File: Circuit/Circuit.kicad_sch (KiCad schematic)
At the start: 26 parts, among them J1 Conn_01x08_Socket, J2 Conn_01x08_Socket, Q2 S8050, Q3 S8050, Q4 S8550, Q5 IRFZ44n, SW1 SW_DPDT_x2, SW2 SW_DPDT_x2, U1 L7805

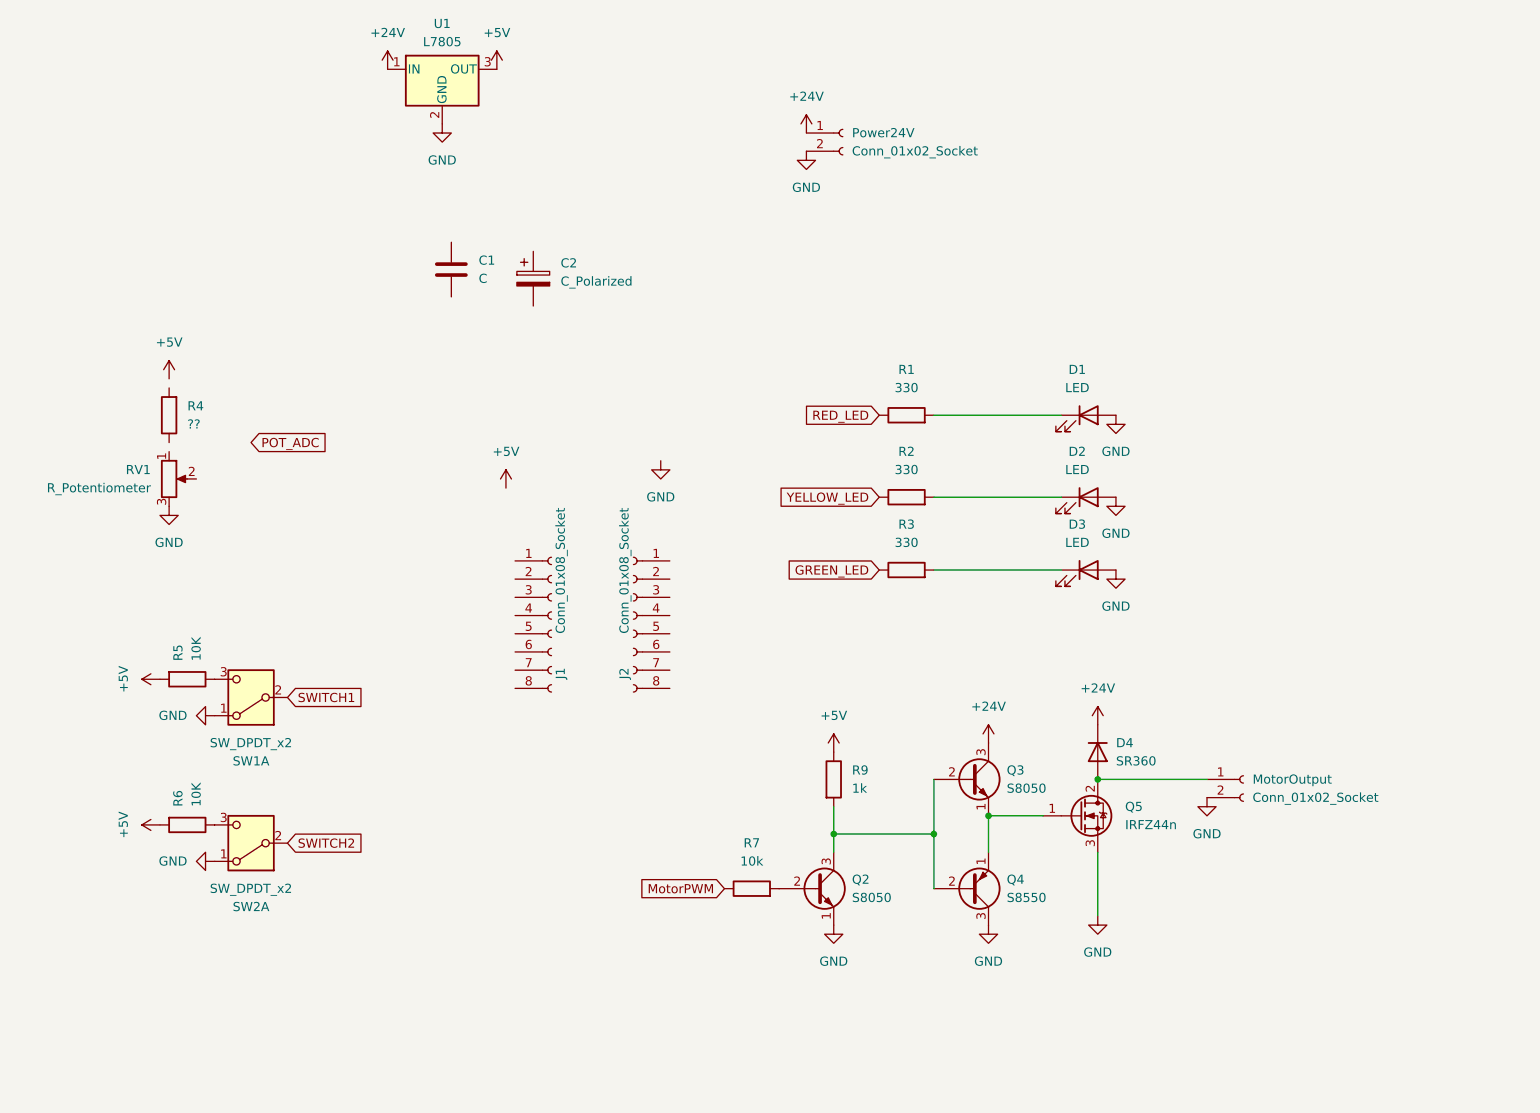
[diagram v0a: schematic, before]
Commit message: finished circuit and started PCB
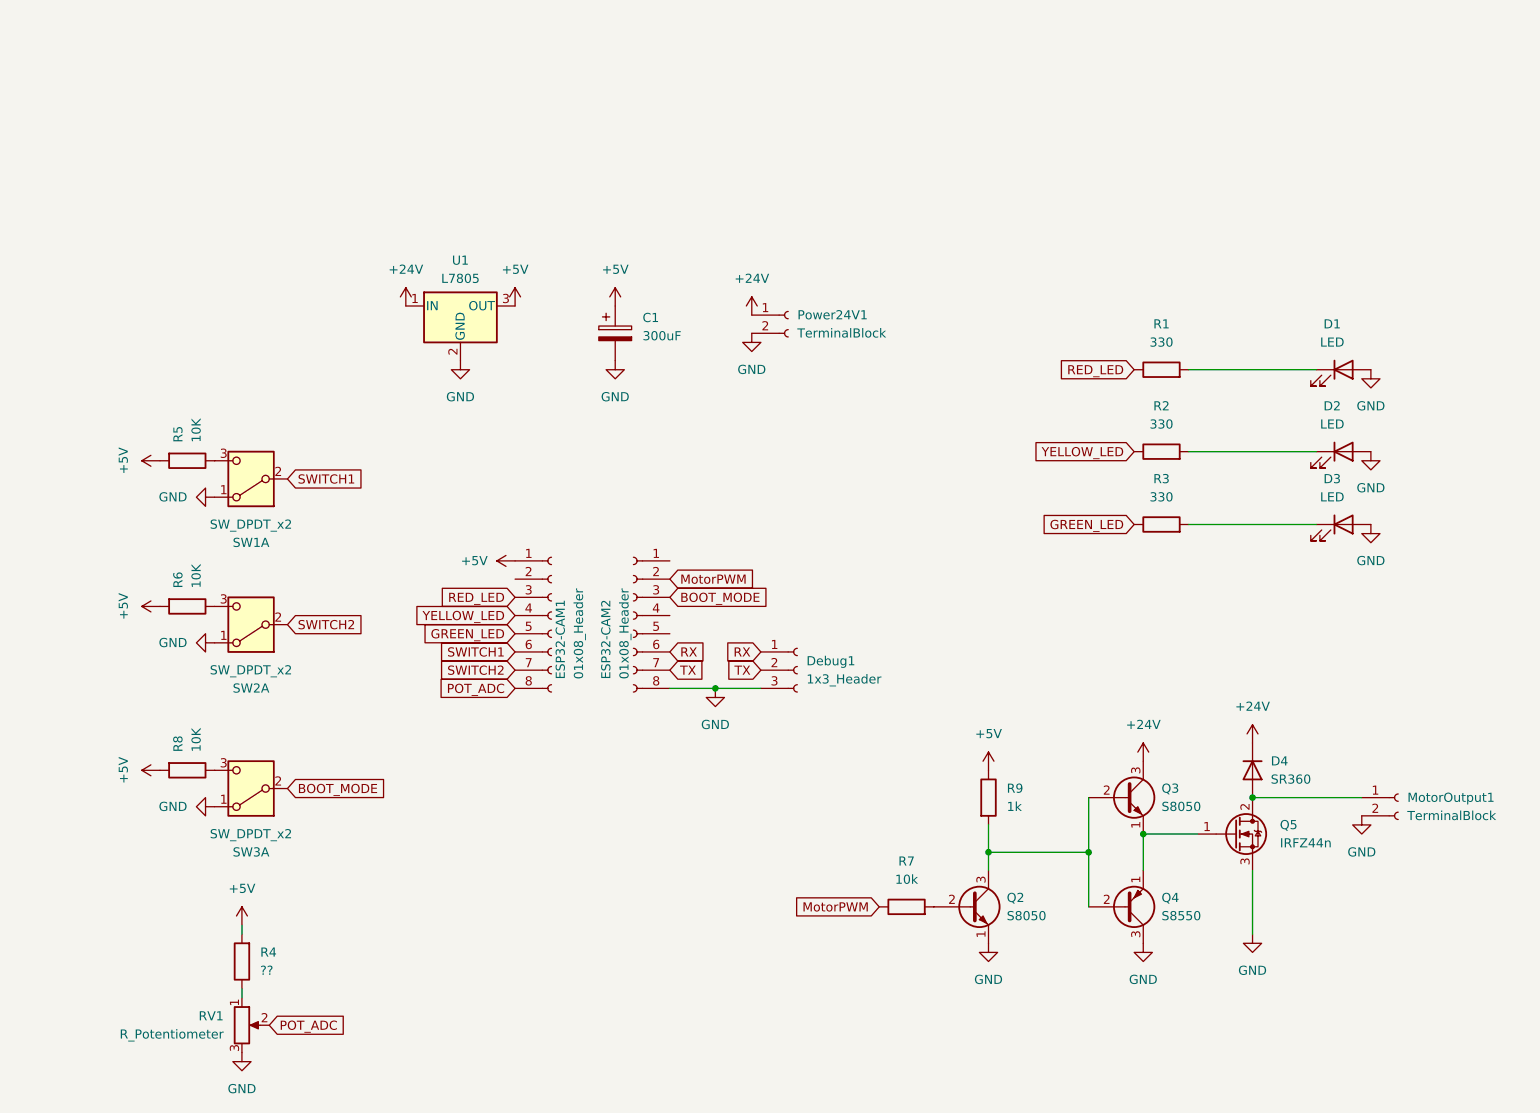
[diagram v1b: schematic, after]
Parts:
- removed C1: C, symbol Device:C
- added Debug1: 1x3_Header, Connector_PinSocket_2.54mm:PinSocket_1x03_P2.54mm_Vertical, symbol Connector:Conn_01x03_Socket
- added R8: 10K, Resistor_THT:R_Axial_DIN0207_L6.3mm_D2.5mm_P7.62mm_Horizontal, symbol Device:R
- added SW3: SW_DPDT_x2, Connector_PinSocket_2.54mm:PinSocket_1x03_P2.54mm_Vertical, symbol Switch:SW_DPDT_x2
- C1: renamed from C2; value C_Polarized -> 300uF; footprint (none) -> Capacitor_THT:CP_Radial_D8.0mm_P3.80mm
- ESP32-CAM1: renamed from J1; value Conn_01x08_Socket -> 01x08_Header
- ESP32-CAM2: renamed from J2; value Conn_01x08_Socket -> 01x08_Header
- MotorOutput1: renamed from MotorOutput; value Conn_01x02_Socket -> TerminalBlock
- Power24V1: renamed from Power24V; value Conn_01x02_Socket -> TerminalBlock
- SW1, SW2: footprint Button_Switch_THT:SW_Slide-03_Wuerth-WS-SLTV_10x2.5x6.4_P2.54mm -> Connector_PinSocket_2.54mm:PinSocket_1x03_P2.54mm_Vertical
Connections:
- net +5V: now also C1.1, ESP32-CAM1.1 (Pin_1), R4.2, R8.2
- net GND: now also C1.2, ESP32-CAM2.8 (Pin_8), Debug1.3 (Pin_3), SW3.1 (A)
- net GREEN_LED: now also ESP32-CAM1.5 (Pin_5)
- net MotorPWM: now also ESP32-CAM2.2 (Pin_2)
- net POT_ADC: now also ESP32-CAM1.8 (Pin_8), RV1.2
- net RED_LED: now also ESP32-CAM1.3 (Pin_3)
- net SWITCH1: now also ESP32-CAM1.6 (Pin_6)
- net SWITCH2: now also ESP32-CAM1.7 (Pin_7)
- net YELLOW_LED: now also ESP32-CAM1.4 (Pin_4)
- net BOOT_MODE: now reaches ESP32-CAM2.3 (Pin_3)
- net BOOT_MODE: now also SW3.2 (B)
- net RX: now reaches ESP32-CAM2.6 (Pin_6)
- net RX: now also Debug1.1 (Pin_1)
- net TX: now reaches ESP32-CAM2.7 (Pin_7)
- net TX: now also Debug1.2 (Pin_2)
- net at RV1.1: now also R4.1
- new net: R8.1, SW3.3 (C)
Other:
- moved on the sheet: C1, D1, D2, D3, D4, MotorOutput1, Power24V1, Q2, Q3, Q4, Q5, R1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
